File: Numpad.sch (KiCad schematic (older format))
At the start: 50 parts, among them SW1 SW_Push, Y1 16MHz

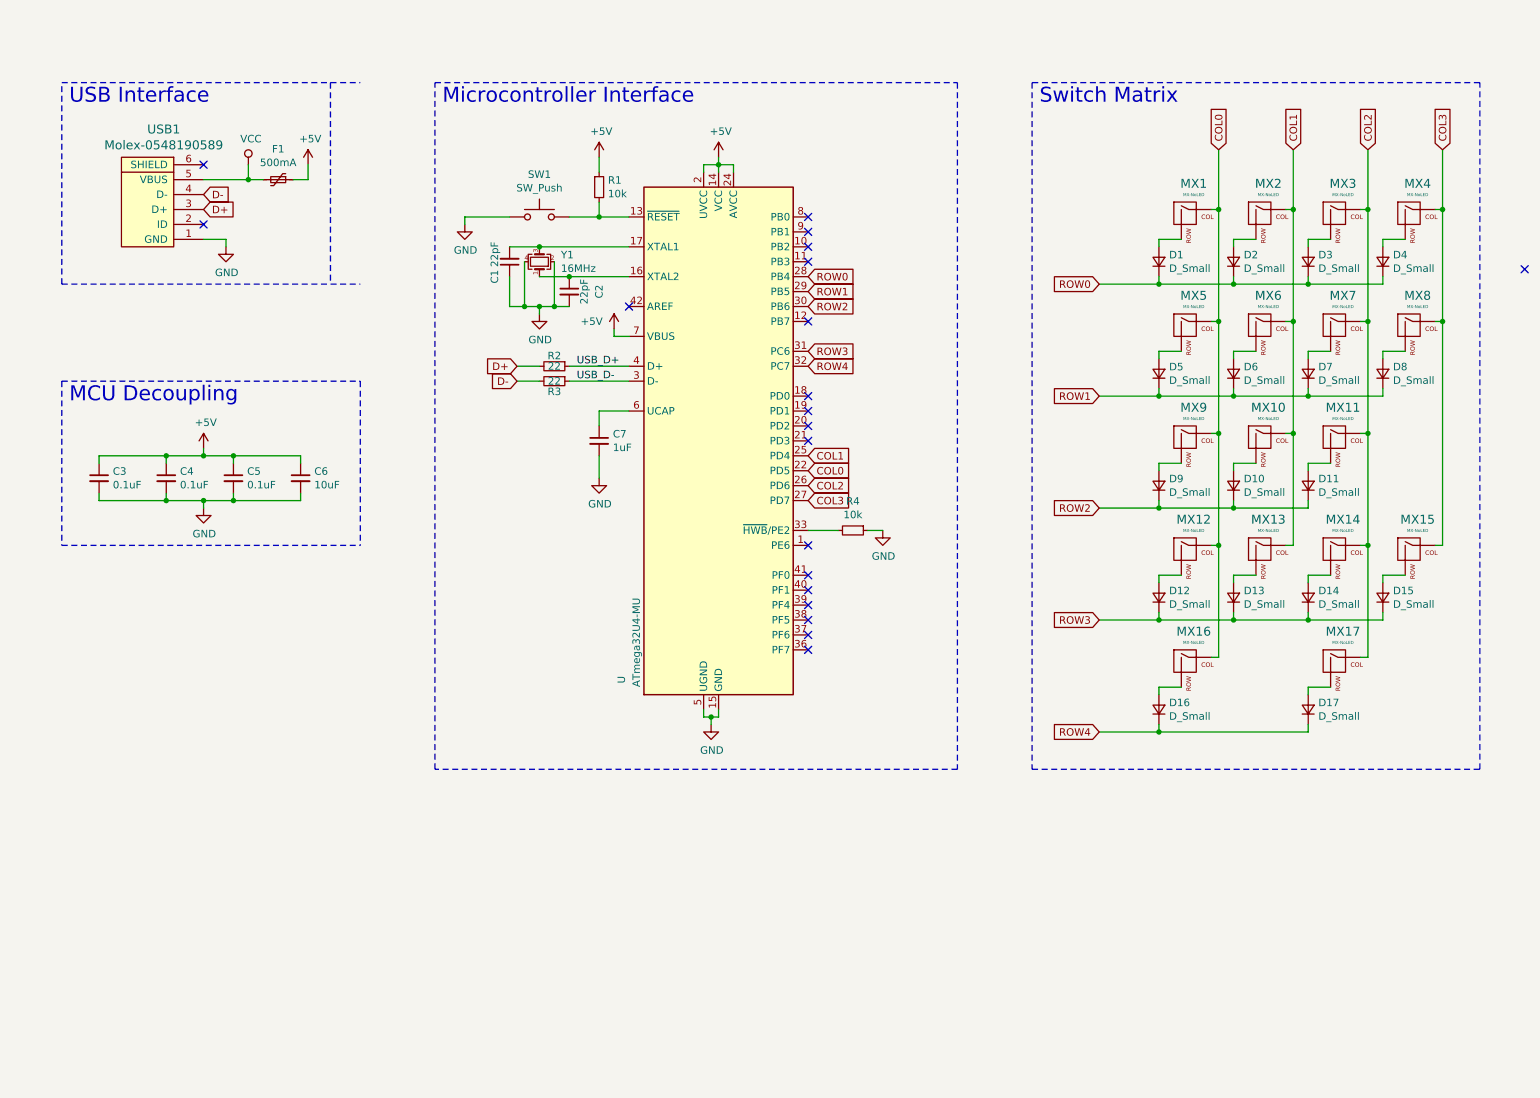
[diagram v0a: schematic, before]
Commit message: Restart project
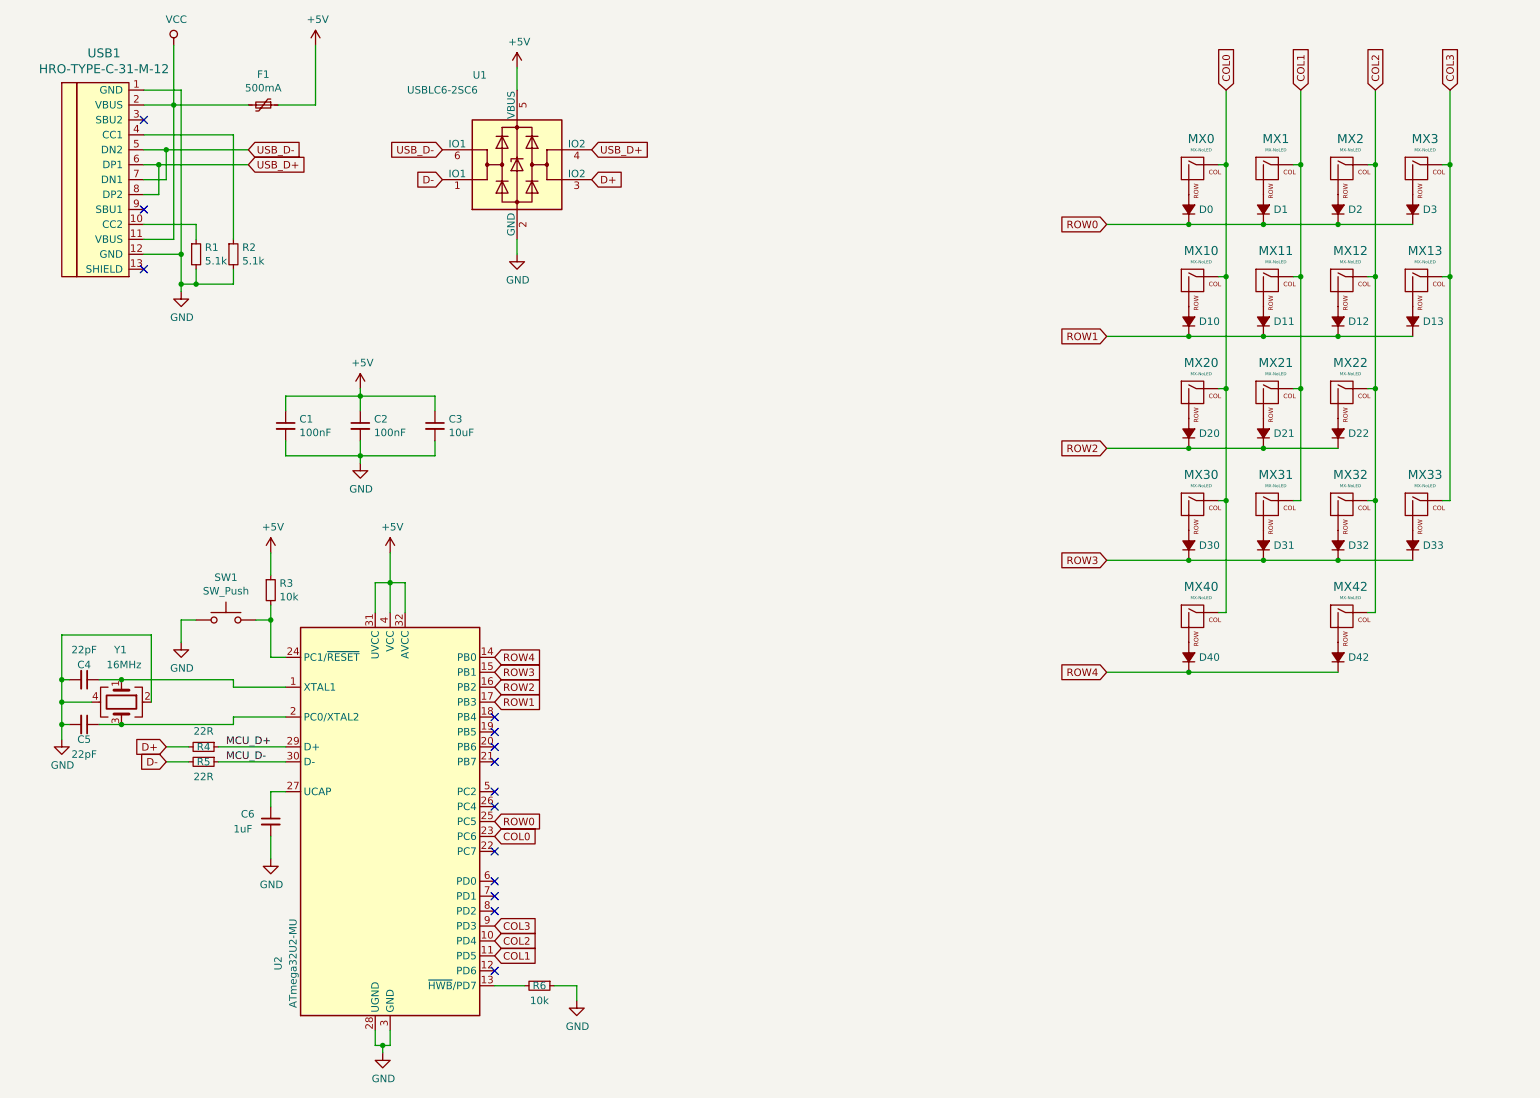
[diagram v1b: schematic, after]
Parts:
- removed C7: 1uF, Capacitor_SMD:C_1206_3216Metric, symbol Device:C_Small
- removed D1, D10, D11, D12, D13, D14, D15, D16, D17, D2, D3, D4, D5, D6, D7, D8, D9: D_Small, Diode_SMD:D_SOD-123, symbol Device:D_Small
- removed MX14, MX17, MX4, MX5, MX6, MX7, MX9: MX-NoLED, MX_Alps_Hybrid:MX-1U-NoLED, symbol MX_Alps_Hybrid:MX-NoLED
- removed MX15, MX8: MX-NoLED, MX_Alps_Hybrid:MX-2U-ReversedStabilizers-Vertical-NoLED, symbol MX_Alps_Hybrid:MX-NoLED
- removed MX16: MX-NoLED, MX_Alps_Hybrid:MX-2U-ReversedStabilizers-NoLED, symbol MX_Alps_Hybrid:MX-NoLED
- removed U: ATmega32U4-MU, Package_DFN_QFN:QFN-44-1EP_7x7mm_P0.5mm_EP5.2x5.2mm, symbol MCU_Microchip_ATmega:ATmega32U4-MU
- removed USB1: Molex-0548190589, random-keyboard-parts:Molex-0548190589, symbol random-keyboard-parts:Molex-0548190589
- removed Y1: 16MHz, Crystal:Crystal_SMD_3225-4Pin_3.2x2.5mm, symbol Device:Crystal_GND24_Small
- added D0, D1, D10, D11, D12, D13, D2, D20, D21, D22, D3, D30, D31, D32, D33, D40, D42: D_Small_ALT, Diode_SMD:D_SOD-123, symbol Device:D_Small_ALT
- added MX0, MX20, MX21, MX22, MX30, MX31, MX32, MX42: MX-NoLED, MX_Only:MXOnly-1U-NoLED, symbol MX_Alps_Hybrid:MX-NoLED
- added MX33, MX40: MX-NoLED, MX_Only:MXOnly-2U-ReversedStabilizers-NoLED, symbol MX_Alps_Hybrid:MX-NoLED
- added R5: 22R, Resistor_SMD:R_0402_1005Metric, symbol Device:R_Small
- added R6: 10k, Resistor_SMD:R_0402_1005Metric, symbol Device:R_Small
- added U1: USBLC6-2SC6, Package_TO_SOT_SMD:SOT-23-6, symbol Power_Protection:USBLC6-2SC6
- added U2: ATmega32U2-MU, Package_DFN_QFN:QFN-32-1EP_5x5mm_P0.5mm_EP3.1x3.1mm, symbol MCU_Microchip_ATmega:ATmega32U2-MU
- added USB1: HRO-TYPE-C-31-M-12, Type-C:HRO-TYPE-C-31-M-12, symbol Type-C:HRO-TYPE-C-31-M-12
- added Y1: 16MHz, Crystal:Crystal_SMD_3225-4Pin_3.2x2.5mm, symbol Device:Crystal_GND24
- C1, C2: value 22pF -> 100nF; footprint Capacitor_SMD:C_1206_3216Metric -> Capacitor_SMD:C_0402_1005Metric; LCSC (none) -> C1525
- C3: value 0.1uF -> 10uF; footprint Capacitor_SMD:C_1206_3216Metric -> Capacitor_SMD:C_0603_1608Metric; LCSC (none) -> C19702
- C4, C5: value 0.1uF -> 22pF; footprint Capacitor_SMD:C_1206_3216Metric -> Capacitor_SMD:C_0402_1005Metric; LCSC (none) -> C1555
- C6: value 10uF -> 1uF; footprint Capacitor_SMD:C_1206_3216Metric -> Capacitor_SMD:C_0402_1005Metric; LCSC (none) -> C52923
- F1: footprint Fuse:Fuse_1206_3216Metric -> Fuse:Fuse_0603_1608Metric; LCSC (none) -> C261937
- MX1, MX10, MX11, MX12, MX2, MX3: footprint MX_Alps_Hybrid:MX-1U-NoLED -> MX_Only:MXOnly-1U-NoLED
- MX13: footprint MX_Alps_Hybrid:MX-1U-NoLED -> MX_Only:MXOnly-2U-ReversedStabilizers-NoLED
- R1: value 10k -> 5.1k; footprint Resistor_SMD:R_0805_2012Metric -> Resistor_SMD:R_0402_1005Metric; LCSC (none) -> C25905
- R2: value 22 -> 5.1k; footprint Resistor_SMD:R_0805_2012Metric -> Resistor_SMD:R_0402_1005Metric; LCSC (none) -> C25905
- R3: value 22 -> 10k; footprint Resistor_SMD:R_0805_2012Metric -> Resistor_SMD:R_0402_1005Metric; LCSC (none) -> C25744
- R4: value 10k -> 22R; footprint Resistor_SMD:R_0805_2012Metric -> Resistor_SMD:R_0402_1005Metric; LCSC (none) -> C25092
- SW1: footprint random-keyboard-parts:SKQG-1155865 -> Switches:TACTILE_SWITCH_SMD_5.2MM; LCSC (none) -> C318884
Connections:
- net +5V: now also C1.1, C2.1, R3.1, U1.5 (VBUS), U2.31 (UVCC), U2.32 (AVCC), U2.4 (VCC); no longer C4.1, C5.1, C6.1, R1.1
- net COL0: now also MX10.1 (COL), MX0.1 (COL), MX20.1 (COL), MX30.1 (COL), MX40.1 (COL), U2.23 (PC6); no longer MX1.1 (COL), MX12.1 (COL)
- net COL1: now also MX1.1 (COL), MX11.1 (COL), MX21.1 (COL), MX31.1 (COL), U2.11 (PD5); no longer MX10.1 (COL), MX13.1 (COL), MX2.1 (COL)
- net COL2: now also MX12.1 (COL), MX2.1 (COL), MX22.1 (COL), MX32.1 (COL), MX42.1 (COL), U2.10 (PD4); no longer MX11.1 (COL), MX3.1 (COL)
- net COL3: now also MX13.1 (COL), MX3.1 (COL), MX33.1 (COL), U2.9 (PD3)
- net D+: now also R4.2, U1.3 (IO2); no longer R2.2
- net D-: now also R5.2, U1.1 (IO1); no longer R3.2
- net GND: now also C1.2, R1.2, R2.2, R6.1, U1.2 (GND), U2.28 (UGND), U2.3 (GND), U2.33 (GND), USB1.1 (GND), USB1.12 (GND), Y1.2, Y1.4; no longer C1.1, R4.1
- net ROW0: now also D0.1 (K), D1.1 (K), D2.1 (K), D3.1 (K), U2.25 (PC5)
- net ROW1: now also D10.1 (K), D11.1 (K), D12.1 (K), D13.1 (K), U2.17 (PB3)
- net ROW2: now also D20.1 (K), D21.1 (K), D22.1 (K), U2.16 (PB2)
- net ROW3: now also D30.1 (K), D31.1 (K), D32.1 (K), D33.1 (K), U2.15 (PB1)
- net ROW4: now also D40.1 (K), D42.1 (K), U2.14 (PB0)
- net USB_D+: now also U1.4 (IO2), USB1.6 (DP1), USB1.8 (DP2); no longer R2.1
- net USB_D-: now also U1.6 (IO1), USB1.5 (DN2), USB1.7 (DN1); no longer R3.1
- net VCC: now also USB1.11 (VBUS), USB1.2 (VBUS)
- net at SW1.2: now also R3.2, U2.24 (PC1/~RESET); no longer R1.2
- net at MX1.2 (ROW): now also D1.2 (A)
- net at MX2.2 (ROW): now also D2.2 (A)
- net at MX3.2 (ROW): now also D3.2 (A)
- net at MX10.2 (ROW): now also D10.2 (A)
- net at MX12.2 (ROW): now also D12.2 (A)
- net at MX13.2 (ROW): now also D13.2 (A)
- net at MX11.2 (ROW): now also D11.2 (A)
- new net: D22.2 (A), MX22.2 (ROW)
- new net: D21.2 (A), MX21.2 (ROW)
- new net: D20.2 (A), MX20.2 (ROW)
- new net: D33.2 (A), MX33.2 (ROW)
- new net: D32.2 (A), MX32.2 (ROW)
- new net: D31.2 (A), MX31.2 (ROW)
- new net: D30.2 (A), MX30.2 (ROW)
- new net: D42.2 (A), MX42.2 (ROW)
- new net: D40.2 (A), MX40.2 (ROW)
- new net: D0.2 (A), MX0.2 (ROW)
- new net: R1.1, USB1.10 (CC2)
- new net: R2.1, USB1.4 (CC1)
- new net: C4.1, U2.1 (XTAL1), Y1.1
- new net: R6.2, U2.13 (~HWB~/PD7)
- new net: C5.1, U2.2 (PC0/XTAL2), Y1.3
- new net: C6.1, U2.27 (UCAP)
- new net MCU_D+: R4.1, U2.29 (D+)
- new net MCU_D-: R5.1, U2.30 (D-)
- no-connect marks 20 -> 14
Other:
- note removed: "MCU Decoupling"
- note removed: "Microcontroller Interface"
- note removed: "Switch Matrix"
- note removed: "USB Interface"
